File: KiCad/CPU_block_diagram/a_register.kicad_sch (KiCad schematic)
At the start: 19 parts, among them U7 74LS245, U8 74LS173, U9 74LS173

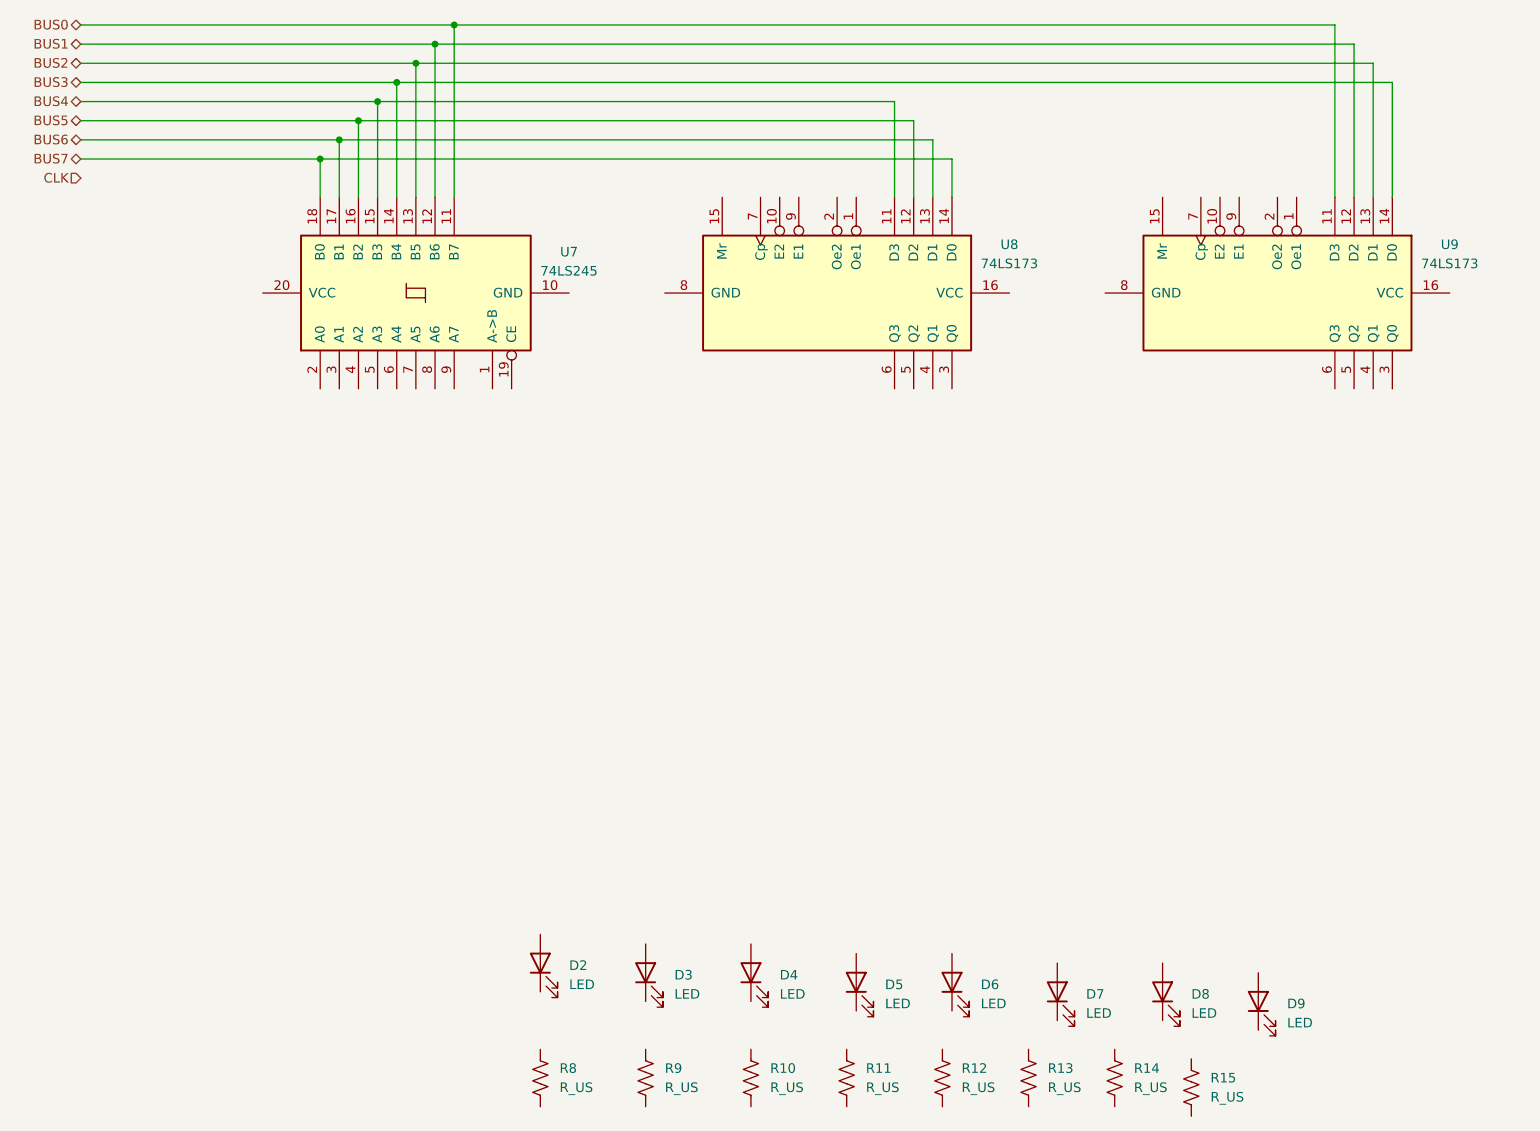
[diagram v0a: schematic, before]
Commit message: vault backup: 2026-01-03 00:49:48
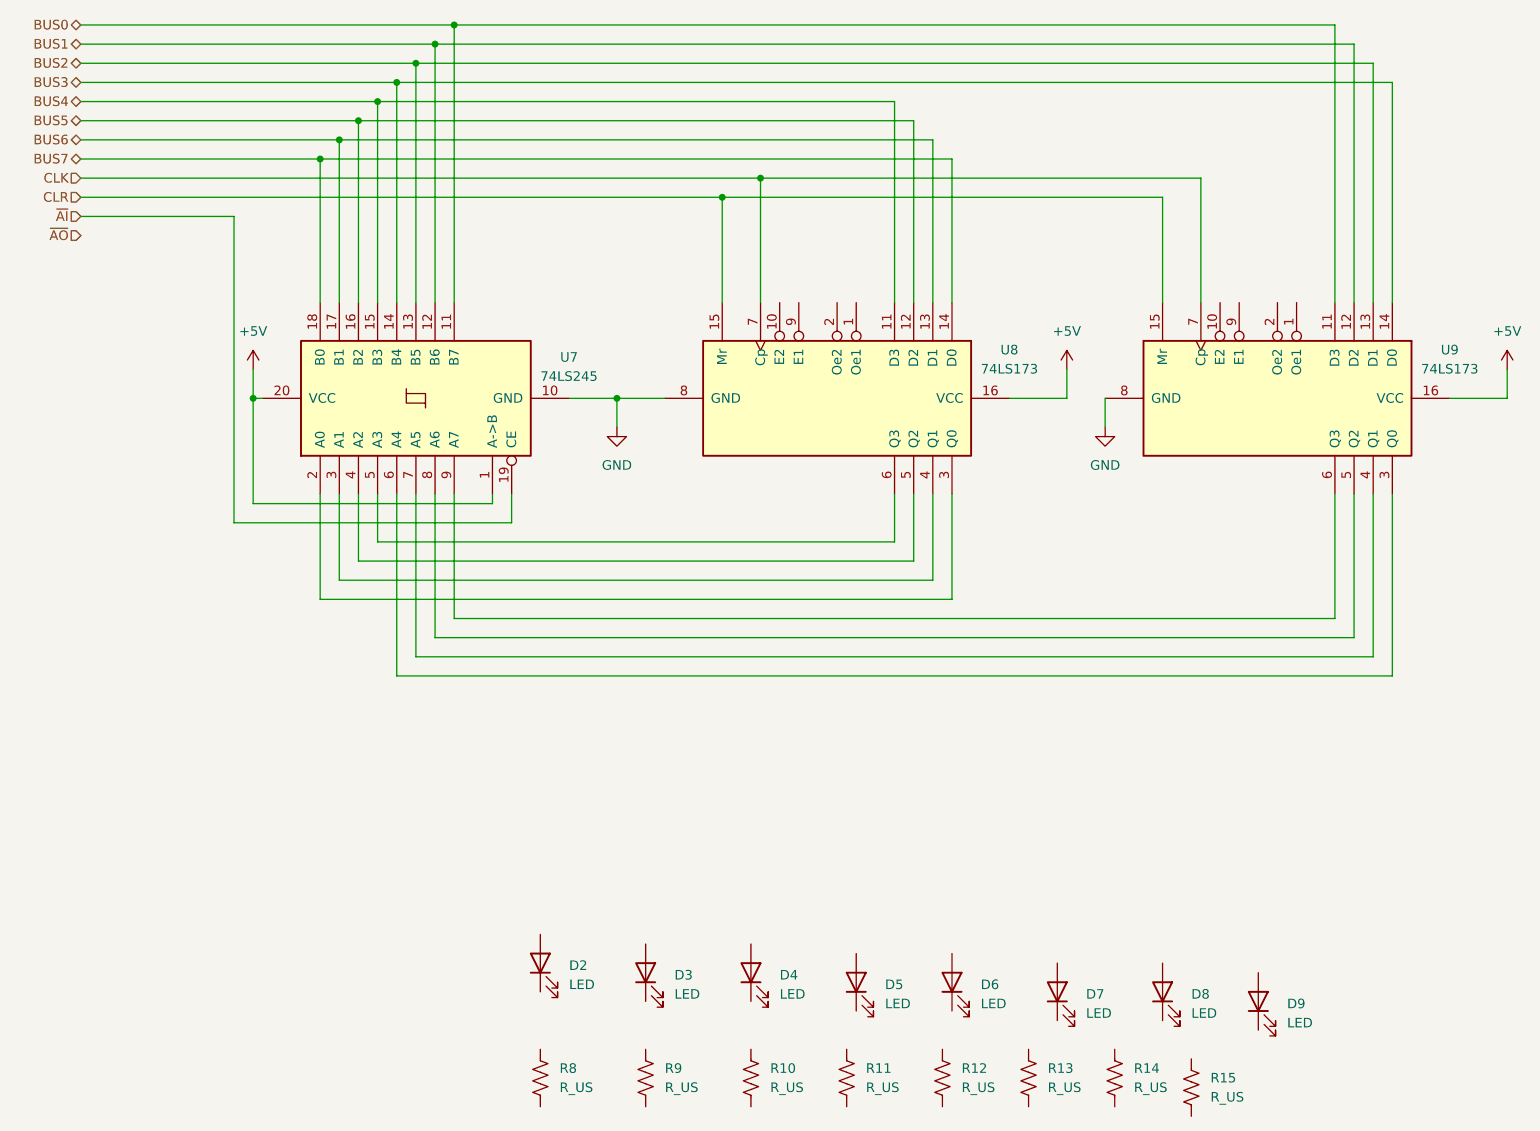
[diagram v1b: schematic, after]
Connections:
- net CLK: now also U8.7 (Cp), U9.7 (Cp)
- net CLR: now reaches U9.15 (Mr)
- net CLR: now also U8.15 (Mr)
- net +5V: now reaches U9.16 (VCC)
- net +5V: now also U7.1 (A->B), U7.20 (VCC), U8.16 (VCC)
- net at U9.3 (Q0): now also U7.6 (A4)
- net at U9.4 (Q1): now also U7.7 (A5)
- net at U9.5 (Q2): now also U7.8 (A6)
- net at U9.6 (Q3): now also U7.9 (A7)
- net GND: now reaches U9.8 (GND)
- net GND: now also U7.10 (GND), U8.8 (GND)
- net at U8.3 (Q0): now also U7.2 (A0)
- net at U8.4 (Q1): now also U7.3 (A1)
- net at U8.5 (Q2): now also U7.4 (A2)
- net at U8.6 (Q3): now also U7.5 (A3)
- net ~{AI}: now reaches U7.19 (CE)
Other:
- moved on the sheet: U7, U8, U9
